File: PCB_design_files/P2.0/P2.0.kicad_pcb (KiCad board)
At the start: 4 copper layers, 18.5 x 18 mm, 58 parts, among them J1 EEG_IN, J2 20021121-00008C4LF, U1 INA819IDRGR, U2 TLV9102, U3 TPS61094, U4 TPS60400, U5 NRF52832-QFAA-R, Y1 32MHz

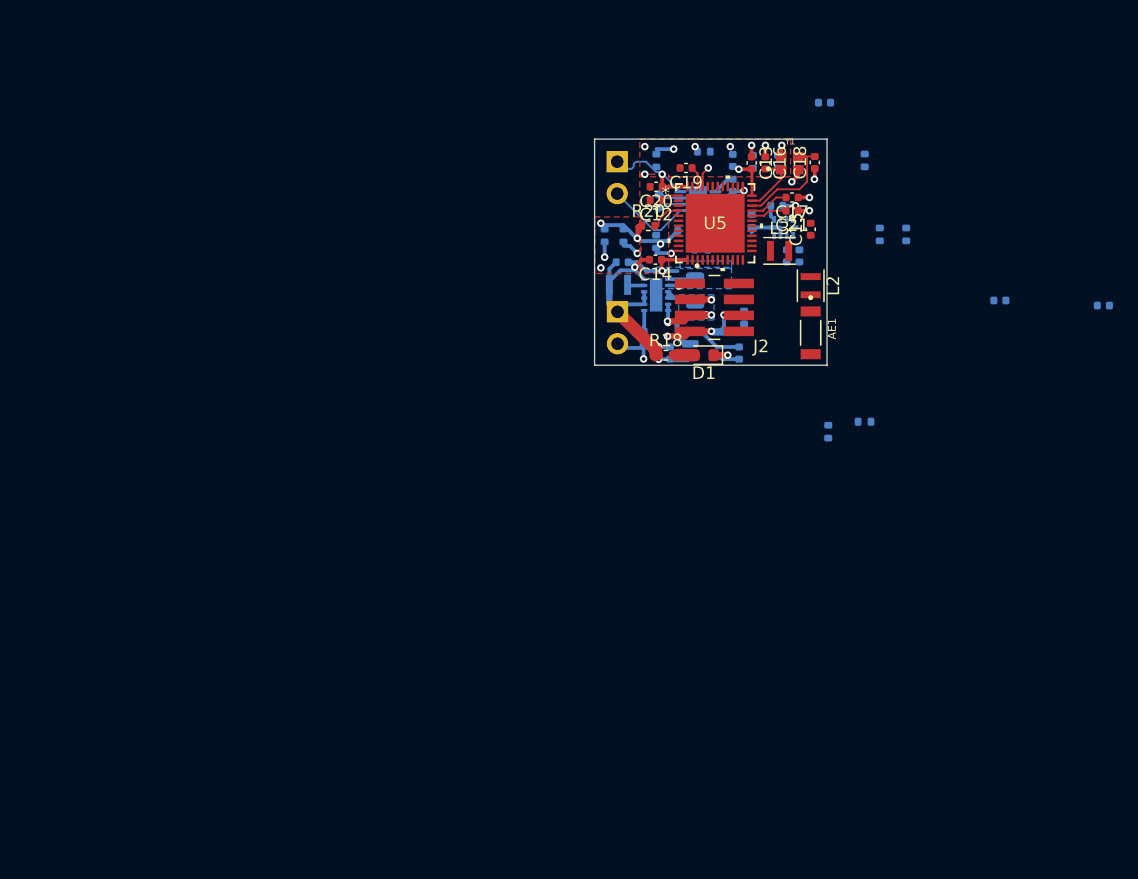
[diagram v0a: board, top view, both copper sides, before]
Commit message: Updated schematic
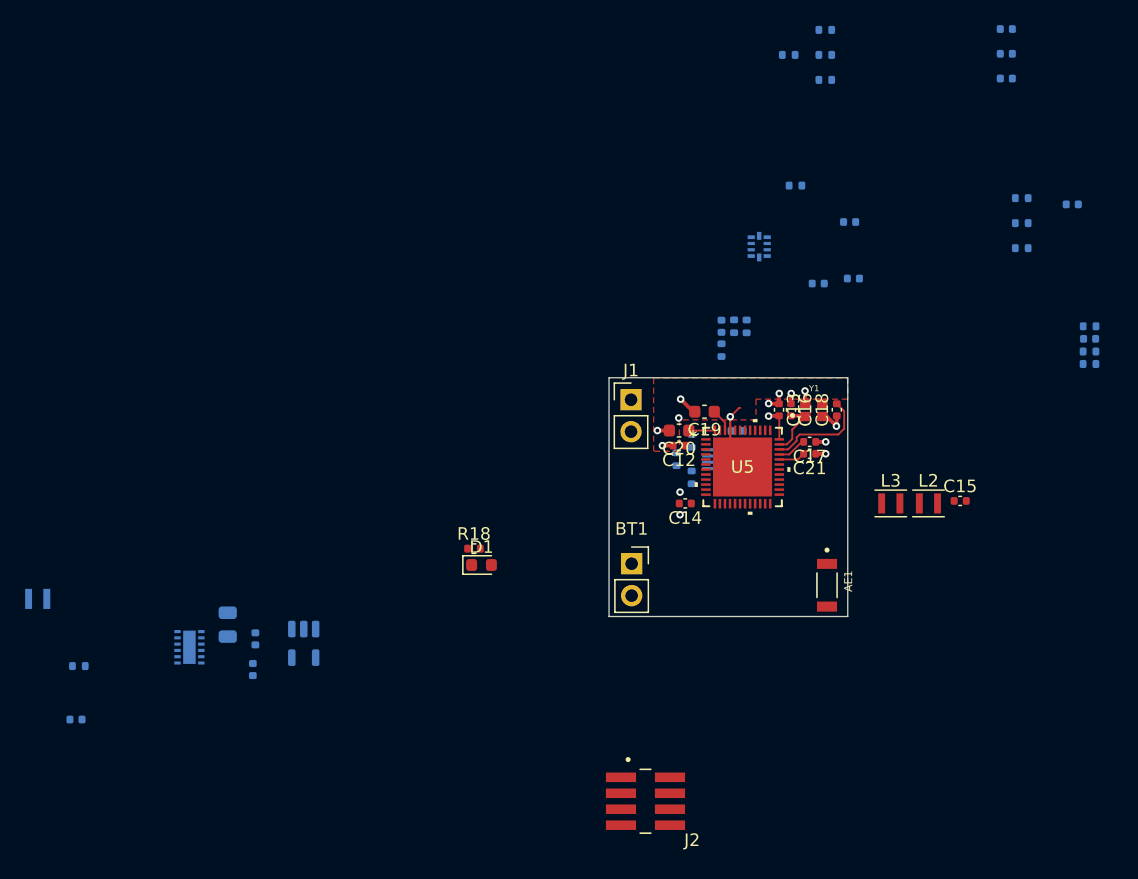
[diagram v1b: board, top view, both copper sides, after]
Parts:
- BT1, J1: moved to F.Cu
- C19, C20: footprint Capacitor_SMD:C_0402_1005Metric -> Capacitor_SMD:C_0603_1608Metric
- R20: moved to B.Cu
- moved C8 56.7 mm to (32.3, 77.2)
- moved L1 52.6 mm to (29.3, 67.6), turned to 180 degrees
- moved R19 52.0 mm to (32.5, 72.9), turned to 180 degrees
- moved U3 46.6 mm to (41.4, 71.5)
- moved C9 45.7 mm to (44.4, 69.7), turned to 90 degrees
- moved C10 44.7 mm to (46.6, 70.8)
- moved C11 41.7 mm to (46.4, 73.2)
- moved R17 39.9 mm to (113.0, 48.9), turned to 180 degrees
- moved U4 39.8 mm to (50.5, 71.1), turned to -90 degrees
- moved J2 39.7 mm to (77.7, 83.7)
- moved R16 38.2 mm to (113.0, 47.9), turned to 0 degrees
- moved C7 33.4 mm to (113.0, 46.9)
- moved R14 31.5 mm to (113.0, 45.9), turned to 0 degrees
- moved R12 30.0 mm to (92.0, 24.3), turned to 180 degrees
- moved R13 27.4 mm to (92.0, 26.3)
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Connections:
- U1 pad 9: (no net) -> -3V3
- U3 pad 13: (no net) -> GND
- U5 pad 49: unconnected-(U5-EPAD-Pad49) -> GND
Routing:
- net GND: track 39.9 -> 20.6 mm, vias 31 -> 13
- net Net-(BT1-+): track 16.2 -> 0.00 mm
- net +3V3: track 21.0 -> 4.83 mm, vias 7 -> 2
- net STAGE_3_OUT: track 7.70 -> 0.00 mm, vias 1 -> 0
- net /EEG+: track 6.87 -> 0.00 mm
- net /EEG-: track 6.62 -> 0.00 mm
- net Net-(U4-CFLY-): track 4.37 -> 0.00 mm
- net -3V3: track 5.62 -> 1.71 mm, vias 1 -> 0
- net Net-(U2-IN1+): track 3.07 -> 0.00 mm
- net Net-(U5-P0.02/AIN0): track 2.35 -> 0.00 mm
- net Net-(R3-Pad2): track 1.94 -> 0.00 mm
- net Net-(R3-Pad1): track 1.94 -> 0.00 mm
- net Net-(U4-CFLY+): track 1.71 -> 0.00 mm
- net Net-(C7-Pad1): track 1.50 -> 0.00 mm
- net Net-(U1-OUT): track 1.44 -> 0.00 mm
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- removed copper zone on B.Cu, net +3V3
- removed copper zone on B.Cu, net GND
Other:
- board size 18.5 x 18 mm -> 19 x 19 mm
